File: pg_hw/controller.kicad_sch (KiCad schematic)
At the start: 27 parts, among them J1 USB_C_Receptacle_USB2.0_14P, J2 Conn_01x03_Pin, J3 Conn_01x03_Pin, Q1 SS8050, Q2 SS8050, SW1 SW_MEC_5E, SW2 SW_MEC_5E, U1 BW16, U2 AMS1117-3.3, U3 CH340C

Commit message: update some things
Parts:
- R1, R2, R3, R4, R5, R6: footprint (none) -> Resistor_SMD:R_0603_1608Metric
- U1: footprint BW16:MODULE_BW16 -> footprints:MODULE_BW16
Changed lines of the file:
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@@
 			)
 		)
-		(property "Footprint" ""
+		(property "Footprint" "Resistor_SMD:R_0603_1608Metric"
 			(at 167.894 30.734 90)
 			(effects
@@
 			)
 		)
-		(property "Footprint" ""
+		(property "Footprint" "Resistor_SMD:R_0603_1608Metric"
 			(at 55.626 118.364 90)
 			(effects
@@
 			)
 		)
-		(property "Footprint" ""
+		(property "Footprint" "Resistor_SMD:R_0603_1608Metric"
 			(at 63.754 35.814 90)
 			(effects
@@
 			)
 		)
-		(property "Footprint" ""
+		(property "Footprint" "Resistor_SMD:R_0603_1608Metric"
 			(at 166.624 47.244 90)
 			(effects
@@
 			)
 		)
-		(property "Footprint" ""
+		(property "Footprint" "Resistor_SMD:R_0603_1608Metric"
 			(at 63.754 38.354 90)
 			(effects
@@
 			)
 		)
-		(property "Footprint" ""
+		(property "Footprint" "Resistor_SMD:R_0603_1608Metric"
 			(at 55.626 141.224 90)
 			(effects
@@
 			)
 		)
-		(property "Footprint" "BW16:MODULE_BW16"
+		(property "Footprint" "footprints:MODULE_BW16"
 			(at 119.38 71.12 0)
 			(effects

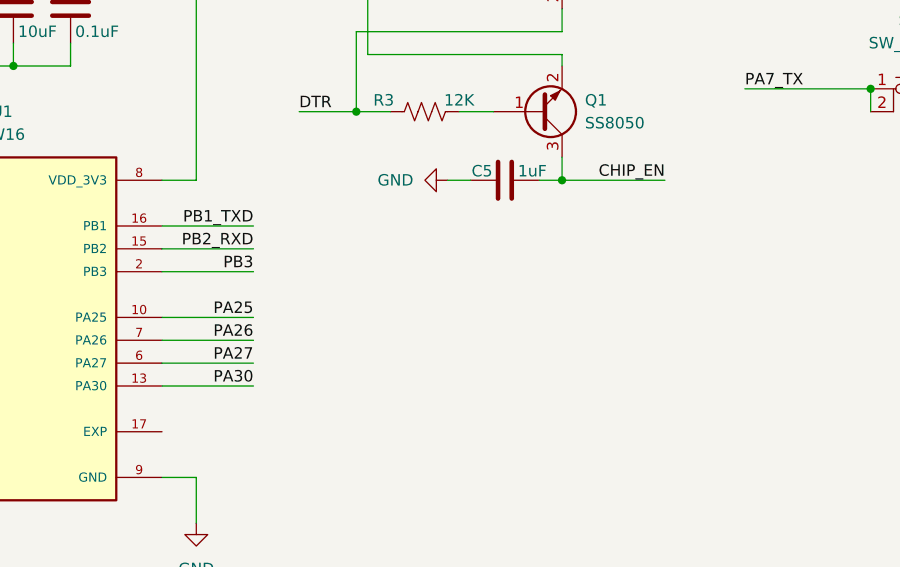
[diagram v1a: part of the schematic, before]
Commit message: change batt again
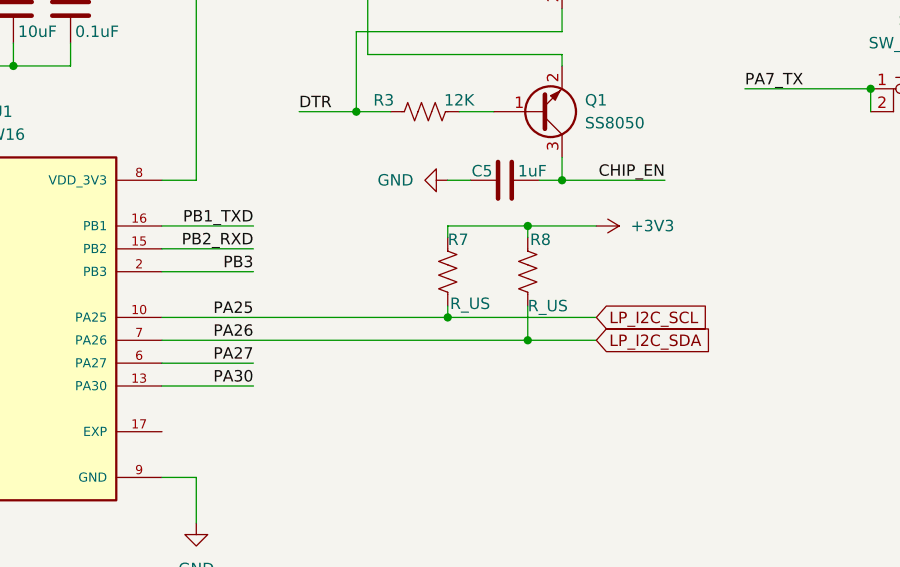
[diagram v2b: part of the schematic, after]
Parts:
- added R7, R8: R_US, symbol Device:R_US
- D5: footprint Diode_THT:D_DO-41_SOD81_P10.16mm_Horizontal -> Diode_SMD:Nexperia_CFP3_SOD-123W
- U3: footprint Package_SO:SOIC-16_3.9x9.9mm_P1.27mm -> Package_SO:SOP-16_3.9x9.9mm_P1.27mm
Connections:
- net +3V3: now also R7.1, R8.1
- net PA25 renamed LP_I2C_SCL
- net LP_I2C_SCL: now also R7.2
- net PA26 renamed LP_I2C_SDA
- net LP_I2C_SDA: now also R8.2

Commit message: hui
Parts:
- C1, C2, C3, C4: footprint (none) -> Resistor_SMD:R_0603_1608Metric
- D5: footprint Diode_SMD:Nexperia_CFP3_SOD-123W -> Diode_THT:D_DO-41_SOD81_P10.16mm_Horizontal
- R3, R4, R5, R6: footprint Resistor_SMD:R_0603_1608Metric -> Resistor_SMD:R_0402_1005Metric
- R7, R8: footprint (none) -> Resistor_SMD:R_0402_1005Metric
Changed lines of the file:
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@@
 			)
 		)
-		(property "Footprint" "Resistor_SMD:R_0603_1608Metric"
+		(property "Footprint" "Resistor_SMD:R_0402_1005Metric"
 			(at 167.894 30.734 90)
 			(effects
@@
 			)
 		)
-		(property "Footprint" ""
+		(property "Footprint" "Resistor_SMD:R_0603_1608Metric"
 			(at 127.9652 40.64 0)
 			(effects
@@
 			)
 		)
-		(property "Footprint" "Resistor_SMD:R_0603_1608Metric"
+		(property "Footprint" "Resistor_SMD:R_0402_1005Metric"
 			(at 55.626 118.364 90)
 			(effects
@@
 			)
 		)
-		(property "Footprint" ""
+		(property "Footprint" "Resistor_SMD:R_0603_1608Metric"
 			(at 92.4052 40.64 0)
 			(effects
@@
 			)
 		)
-		(property "Footprint" "Diode_SMD:Nexperia_CFP3_SOD-123W"
+		(property "Footprint" "Diode_THT:D_DO-41_SOD81_P10.16mm_Horizontal"
 			(at 46.99 126.365 0)
 			(effects
@@
 			)
 		)
-		(property "Footprint" ""
+		(property "Footprint" "Resistor_SMD:R_0402_1005Metric"
 			(at 178.816 66.294 90)
 			(effects
@@
 			)
 		)
-		(property "Footprint" "Resistor_SMD:R_0603_1608Metric"
+		(property "Footprint" "Resistor_SMD:R_0402_1005Metric"
 			(at 166.624 47.244 90)
 			(effects
@@
 			)
 		)
-		(property "Footprint" ""
+		(property "Footprint" "Resistor_SMD:R_0603_1608Metric"
 			(at 121.6152 40.64 0)
 			(effects
@@
 			)
 		)
-		(property "Footprint" "Resistor_SMD:R_0603_1608Metric"
+		(property "Footprint" "Resistor_SMD:R_0402_1005Metric"
 			(at 55.626 141.224 90)
 			(effects
@@
 			)
 		)
-		(property "Footprint" ""
+		(property "Footprint" "Resistor_SMD:R_0402_1005Metric"
 			(at 169.926 66.294 90)
 			(effects
@@
 			)
 		)
-		(property "Footprint" ""
+		(property "Footprint" "Resistor_SMD:R_0603_1608Metric"
 			(at 100.0252 40.64 0)
 			(effects

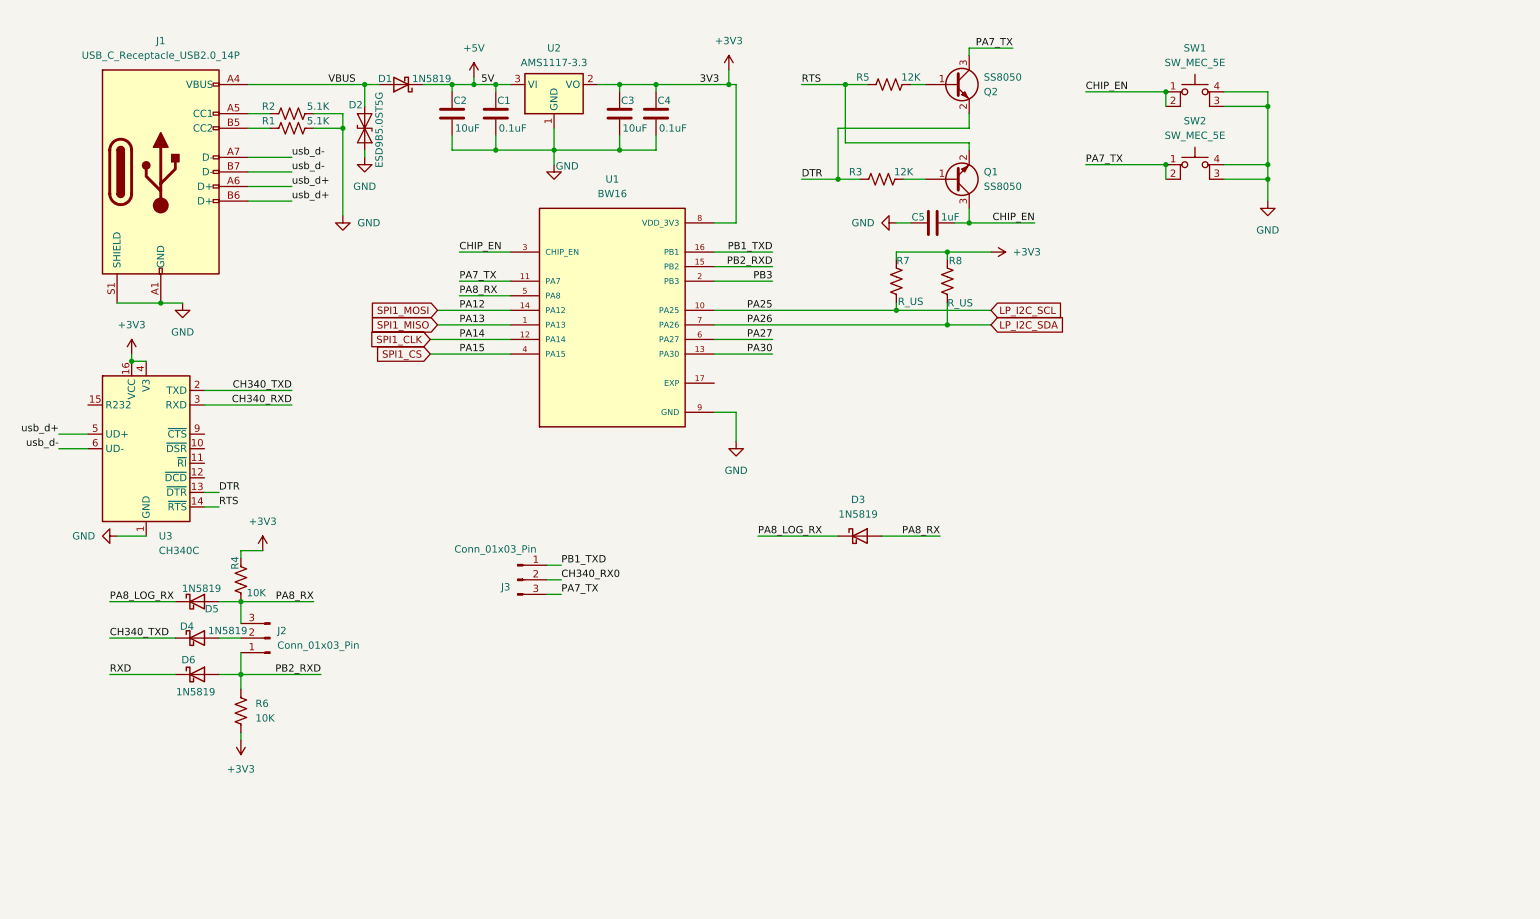
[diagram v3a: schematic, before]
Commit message: push
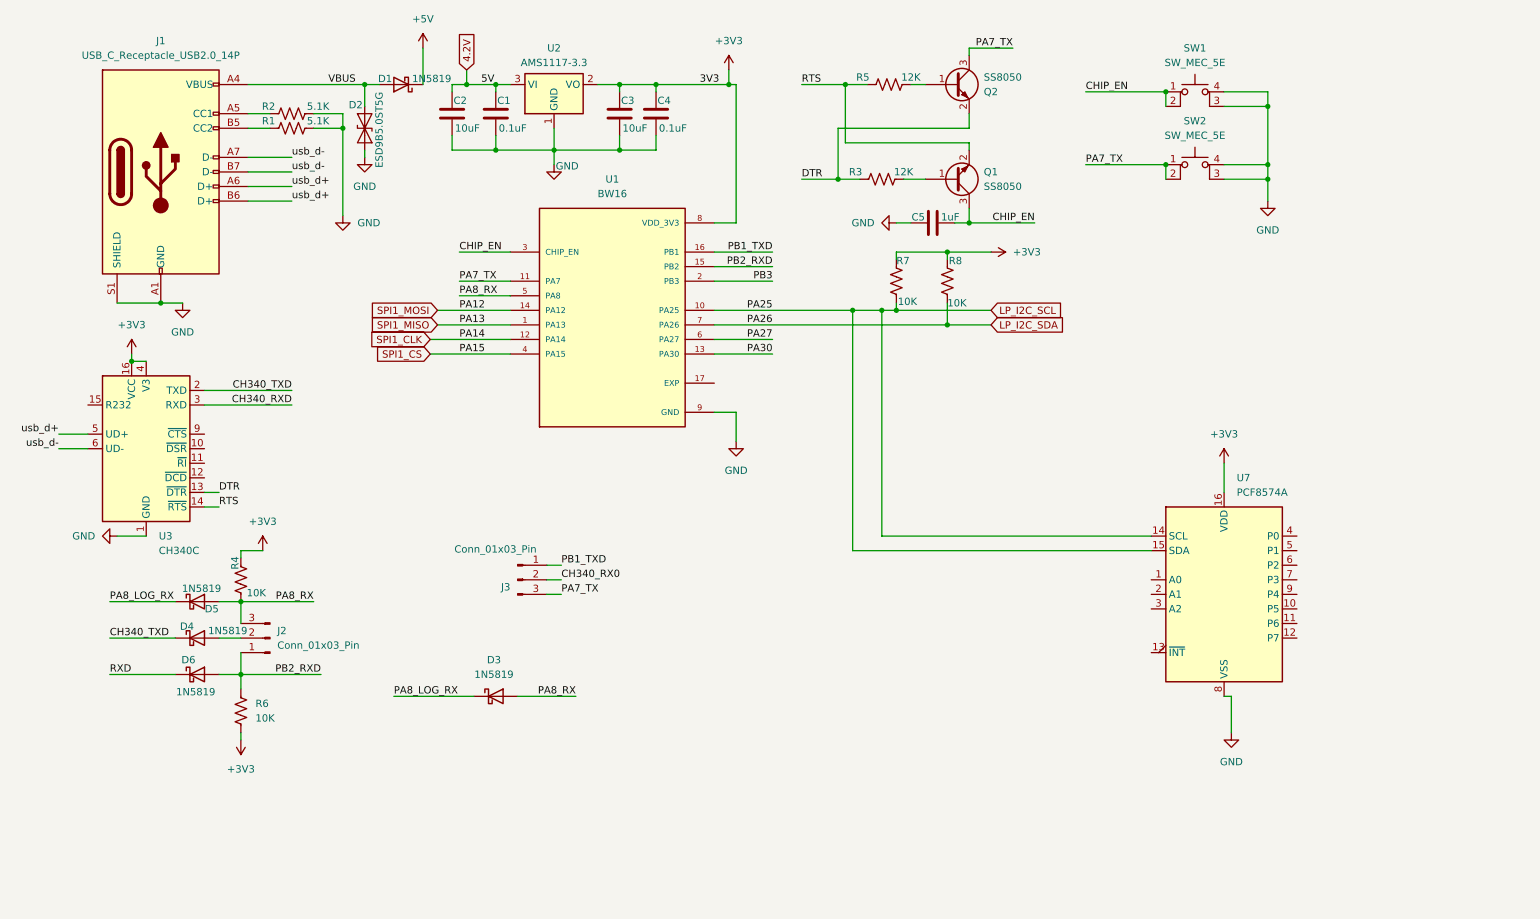
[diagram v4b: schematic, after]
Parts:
- added U7: PCF8574A, symbol Interface_Expansion:PCF8574A
- R7, R8: value R_US -> 10K
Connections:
- net +3V3: now also U7.16 (VDD)
- net +5V: no longer C1.1, C2.1, U2.3 (VI)
- net GND: now also U7.8 (VSS)
- net LP_I2C_SCL: now also U7.14 (SCL), U7.15 (SDA)
- new net 4.2V: C1.1, C2.1, U2.3 (VI)
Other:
- moved on the sheet: D3

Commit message: ADD REV
DADA
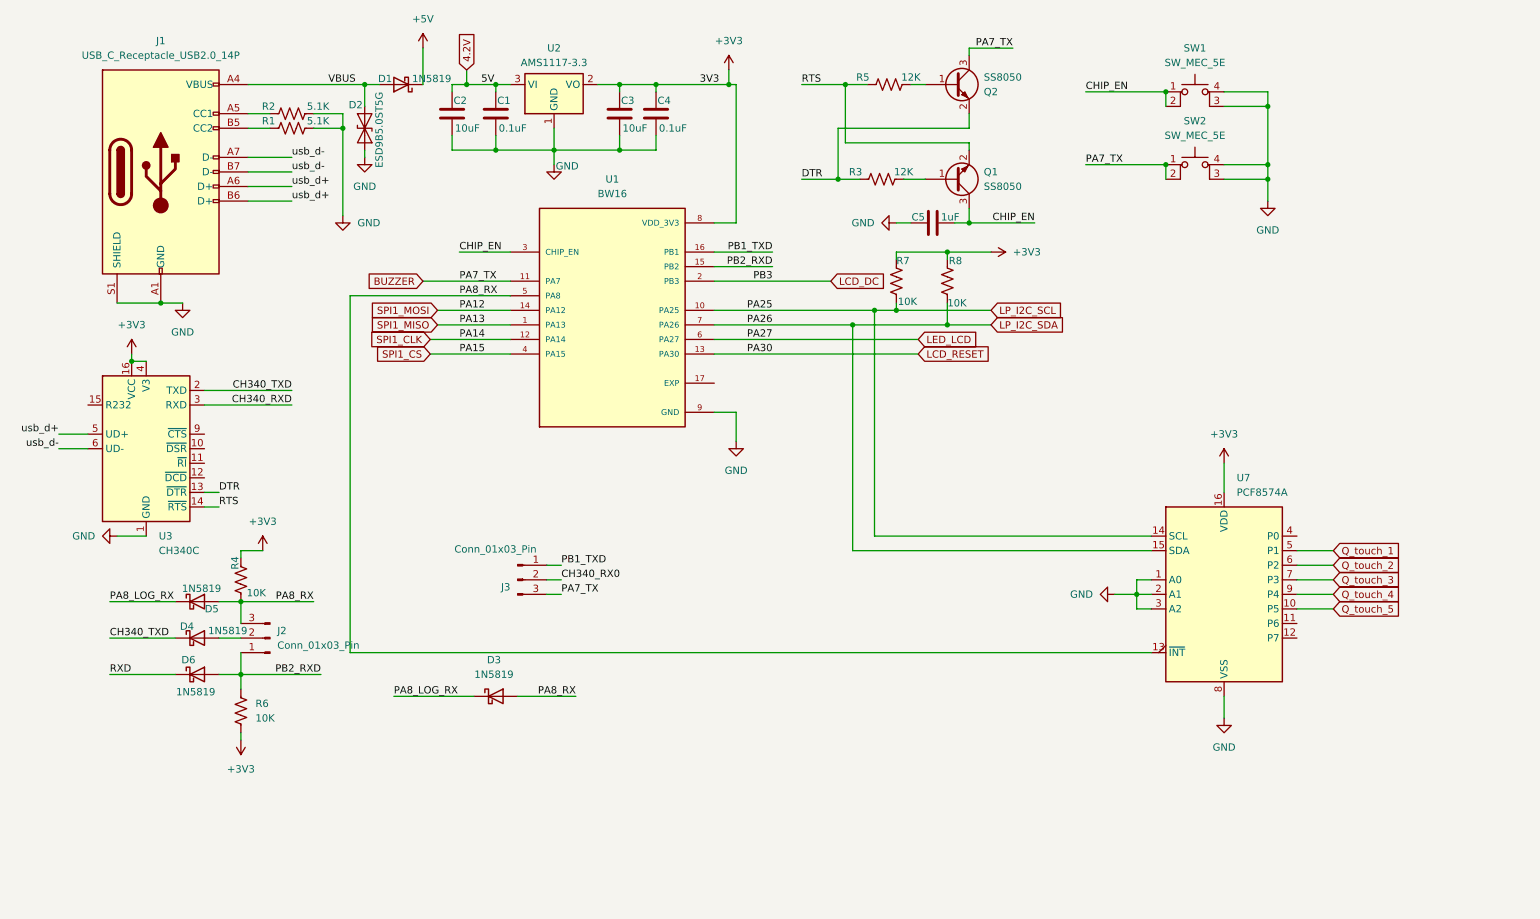
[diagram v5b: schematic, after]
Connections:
- net GND: now also U7.1 (A0), U7.2 (A1), U7.3 (A2)
- net LP_I2C_SCL: no longer U7.15 (SDA)
- net LP_I2C_SDA: now also U7.15 (SDA)
- net PA8_RX: now also U7.13 (~{INT})
- net Q_touch_5: now reaches U7.10 (P5)
- net Q_touch_1: now reaches U7.5 (P1)
- net Q_touch_2: now reaches U7.6 (P2)
- net Q_touch_3: now reaches U7.7 (P3)
- net Q_touch_4: now reaches U7.9 (P4)
- net PA27 renamed LED_LCD
- net PA30 renamed LCD_RESET
- net PA7_TX renamed BUZZER
- net PB3 renamed LCD_DC

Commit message: Mungkin masih akan ada refisi
munvkin
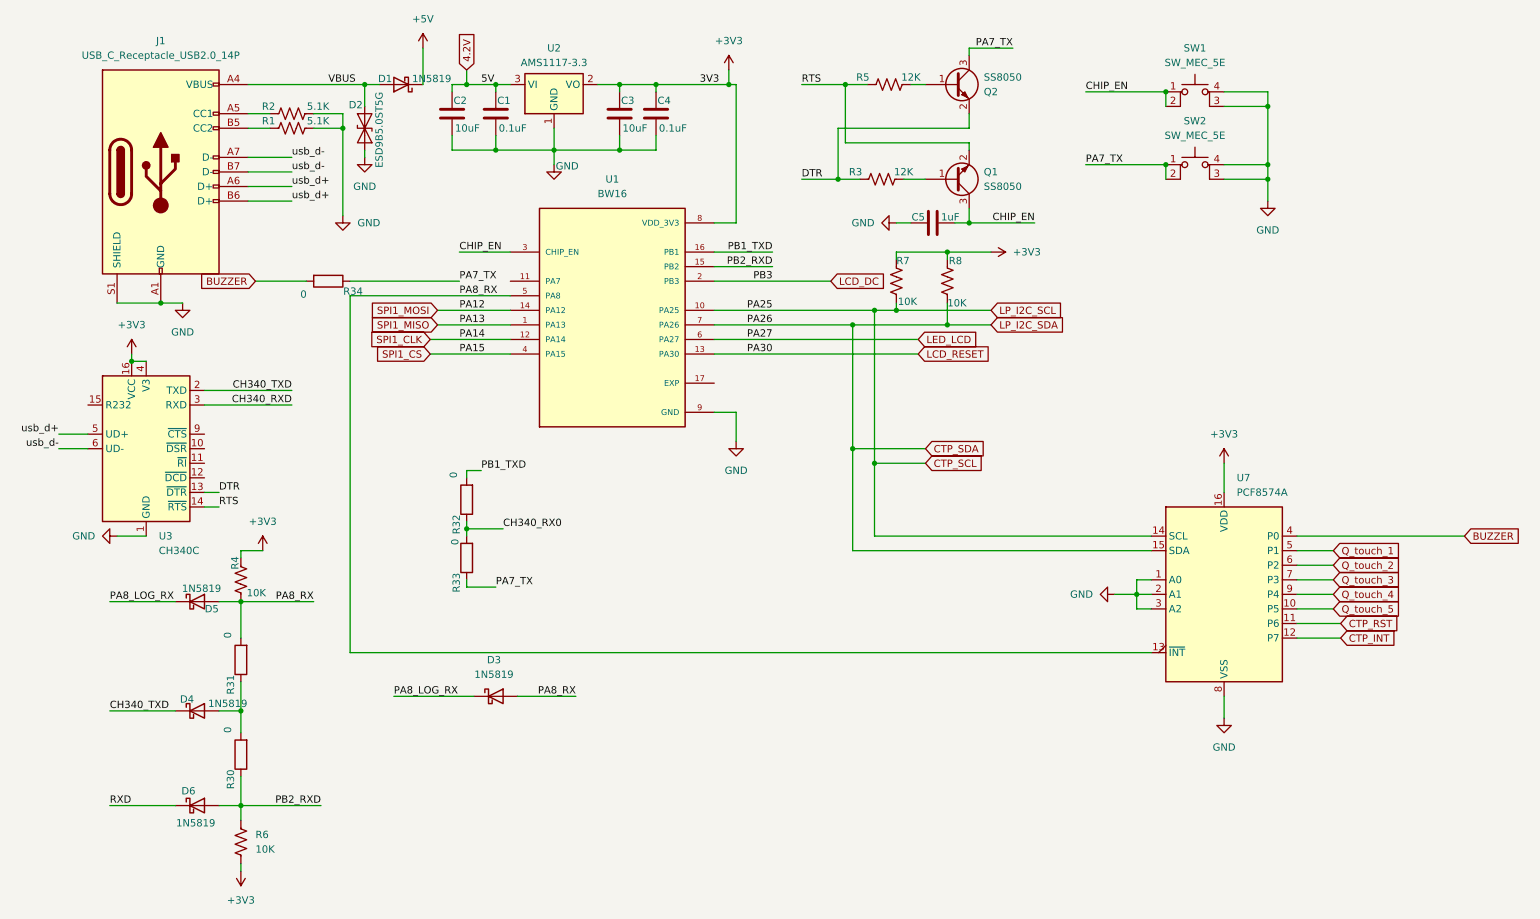
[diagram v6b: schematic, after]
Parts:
- removed J2, J3: Conn_01x03_Pin, symbol Connector:Conn_01x03_Pin
- added R30, R31, R32, R33, R34: 0, symbol Device:R
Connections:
- net BUZZER: now also U7.4 (P0), R34.2; no longer Q2.3 (C), SW2.1, SW2.2, U1.11 (PA7)
- net CH340_RX0: now also R32.1, R33.2
- net PA8_RX: now also R31.2
- net PB1_TXD: now also R32.2
- net PB2_RXD: now also R30.1
- net CTP_RST: now reaches U7.11 (P6)
- net CTP_INT: now reaches U7.12 (P7)
- net at D4.2 (A): now also R30.2, R31.1
- net LP_I2C_SCL renamed CTP_SCL
- net LP_I2C_SDA renamed CTP_SDA
- new net PA7_TX: Q2.3 (C), R33.1, R34.1, SW2.1, SW2.2
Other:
- moved on the sheet: D4, D6, R6
